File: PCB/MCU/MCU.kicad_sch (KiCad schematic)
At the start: 36 parts, among them IC1 TMP112NAIDRLR, J1 Conn_02x06_Odd_Even, J2 Conn_02x06_Odd_Even, J3 USB_B_Micro, J4 Programmer, SW1 SW_Push, U1 MPU6050, U2 MDBT50Q-1MV2, U3 MAX6372, Y1 32.768kHz

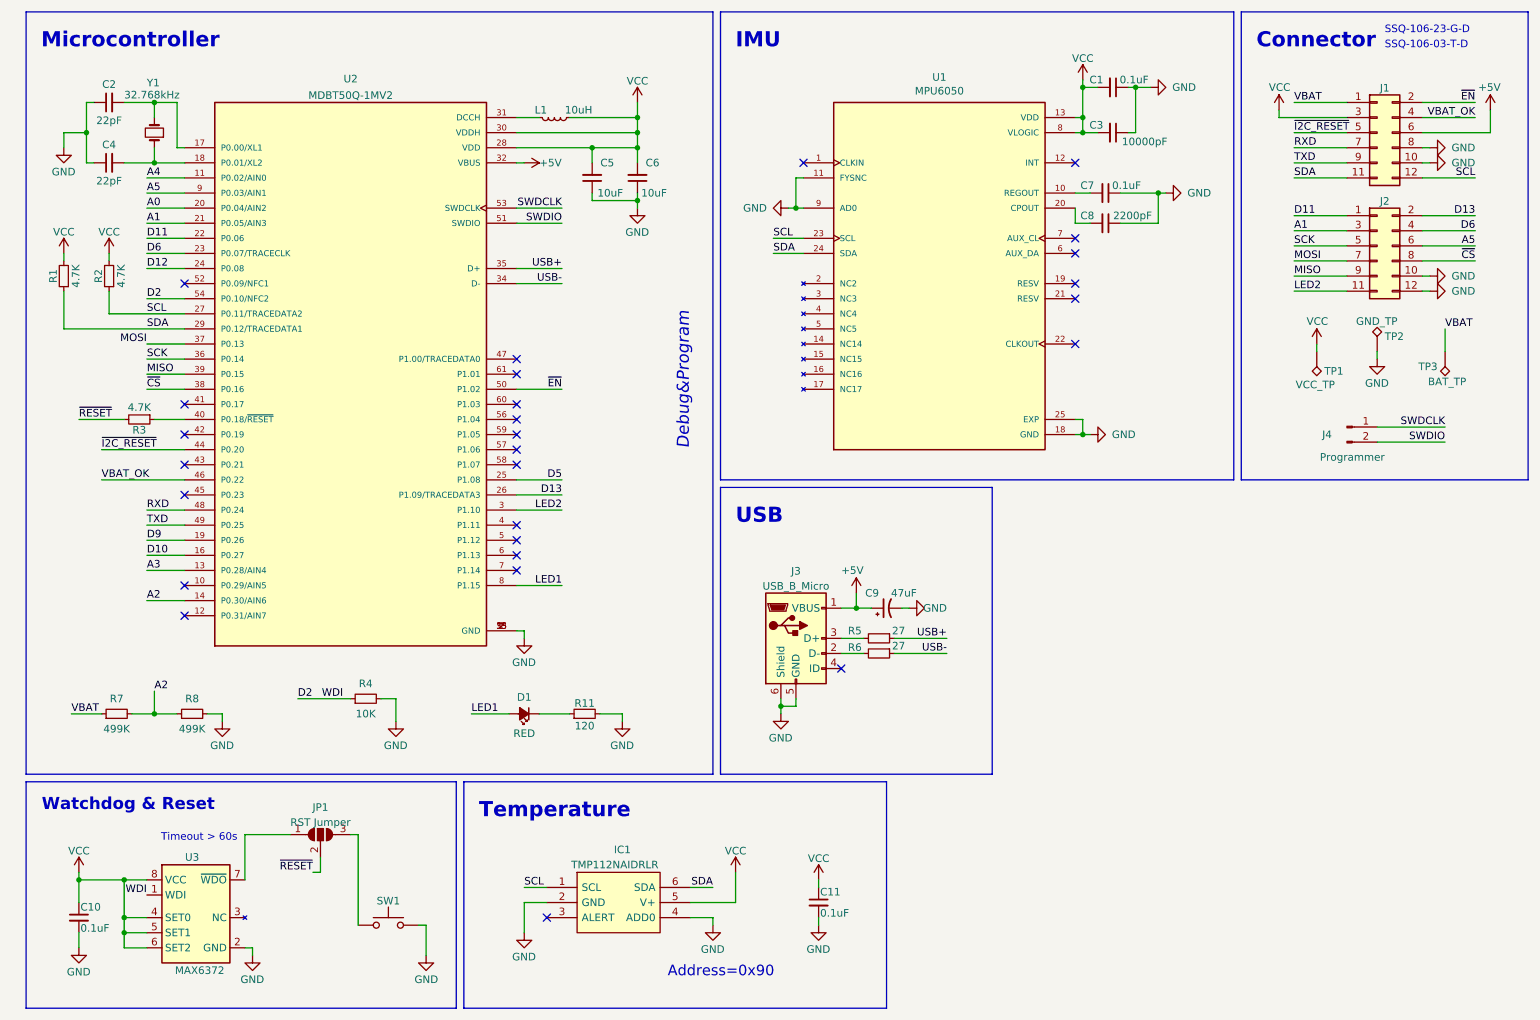
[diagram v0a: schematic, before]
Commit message: udated by FZ from Windows
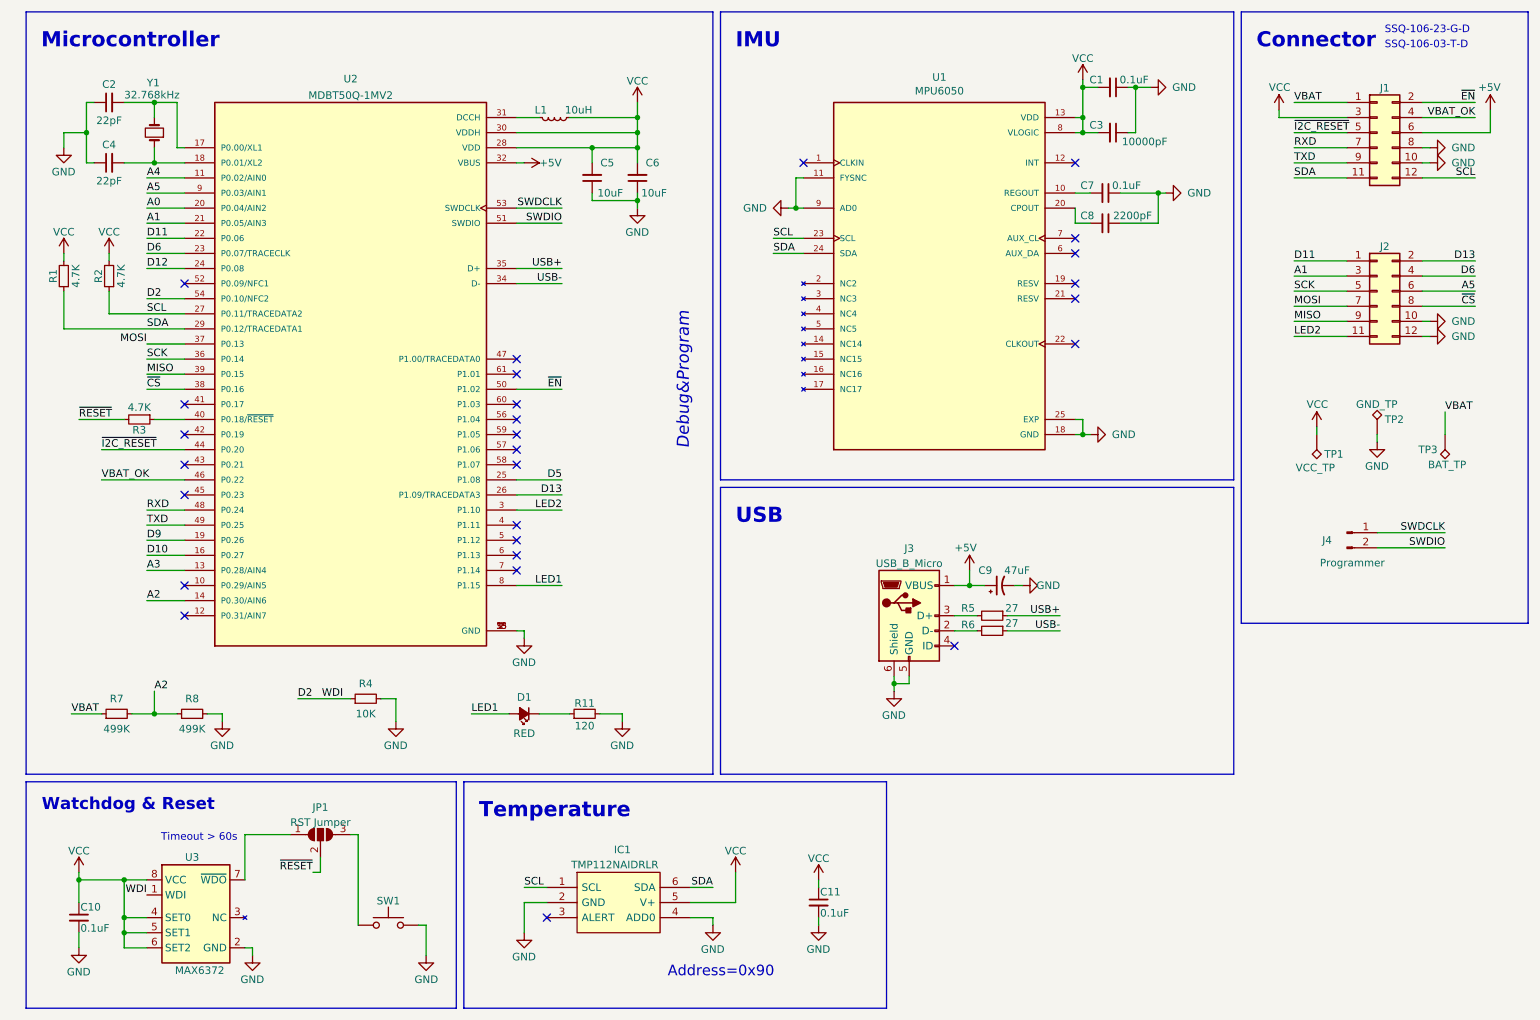
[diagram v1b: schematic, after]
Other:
- moved on the sheet: C9, J2, J3, J4, R5, R6, TP1, TP2, TP3
